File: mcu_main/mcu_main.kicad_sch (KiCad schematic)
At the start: 23 parts, among them SW1 SW_Push_Dual, SW2 SW_Push_Dual, U1 ESP32-S3-WROOM-1, U3 SGM2212-3.3, U5 SGM2212-2.8

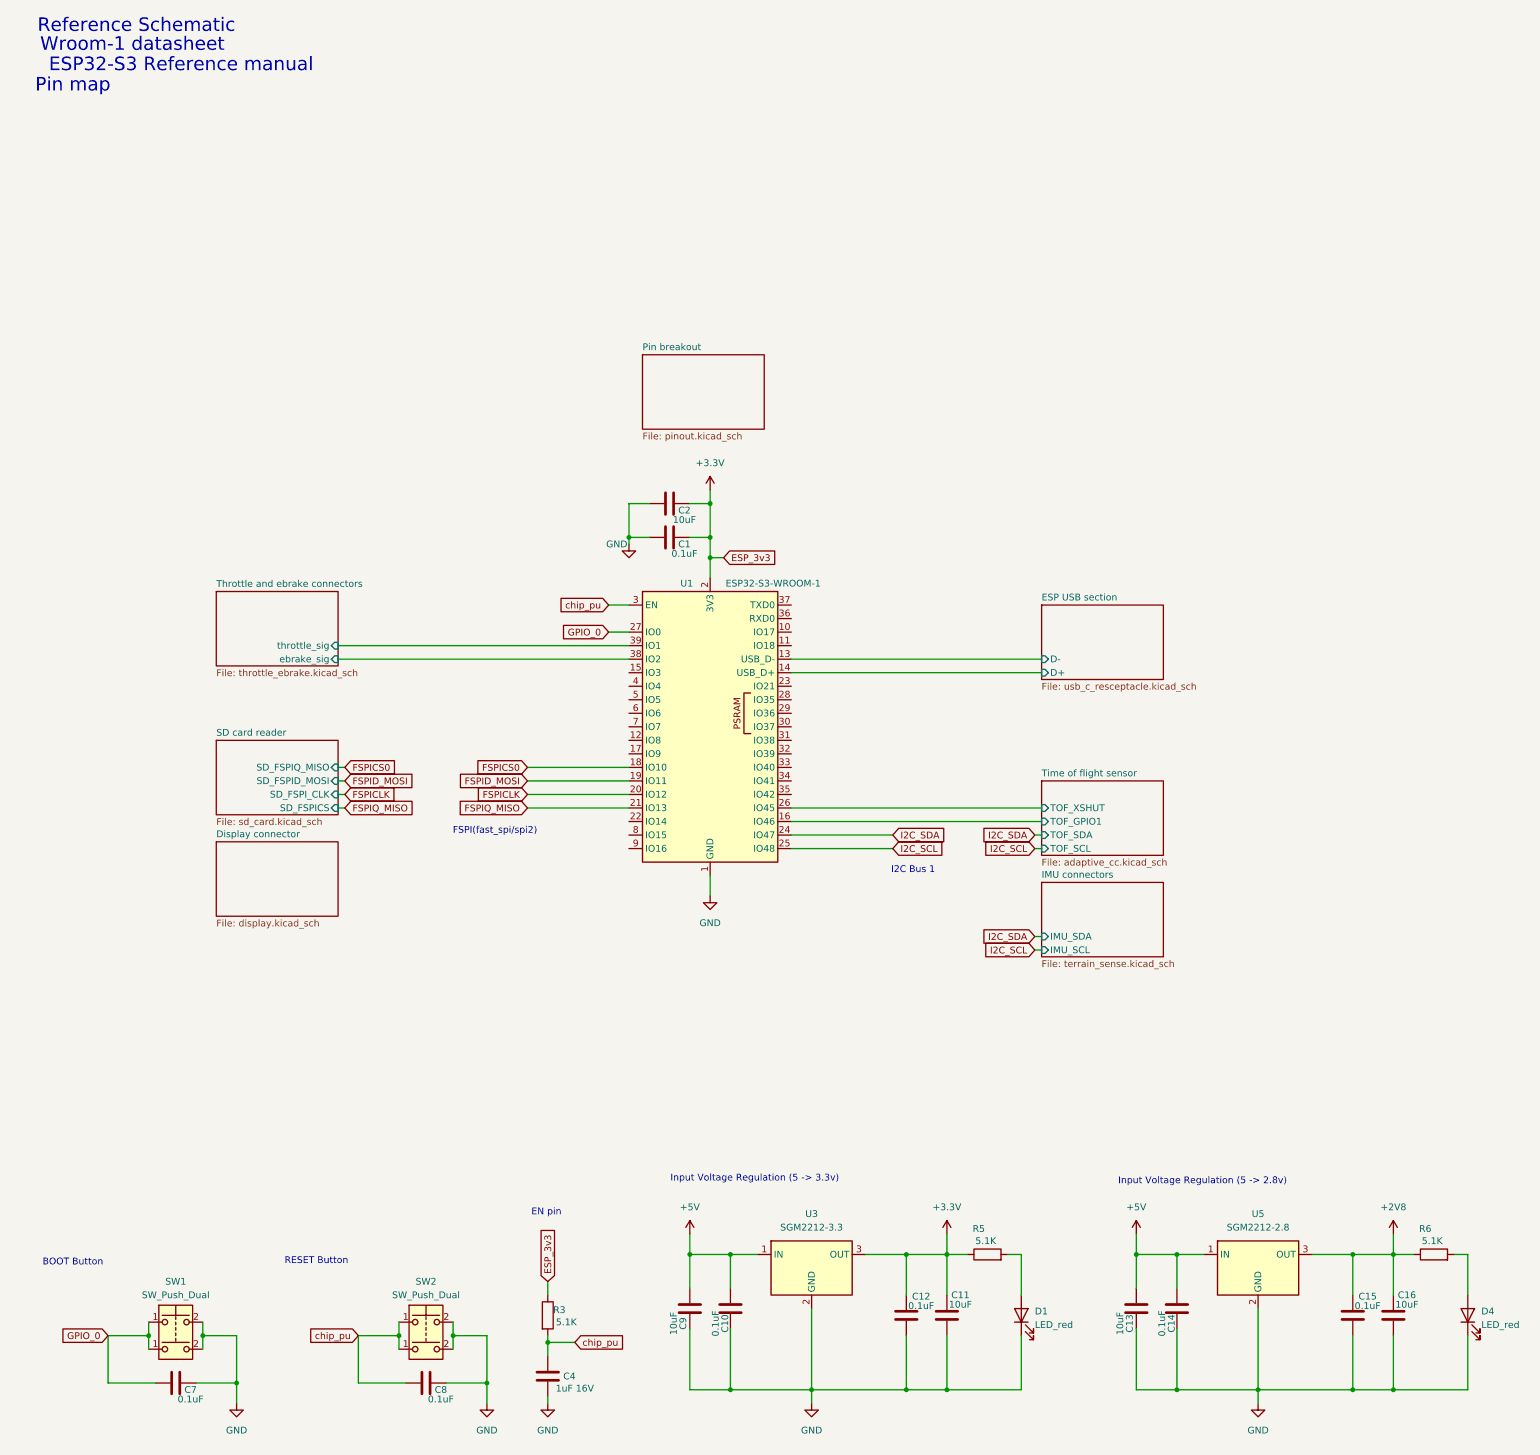
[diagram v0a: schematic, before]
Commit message: pas sensors
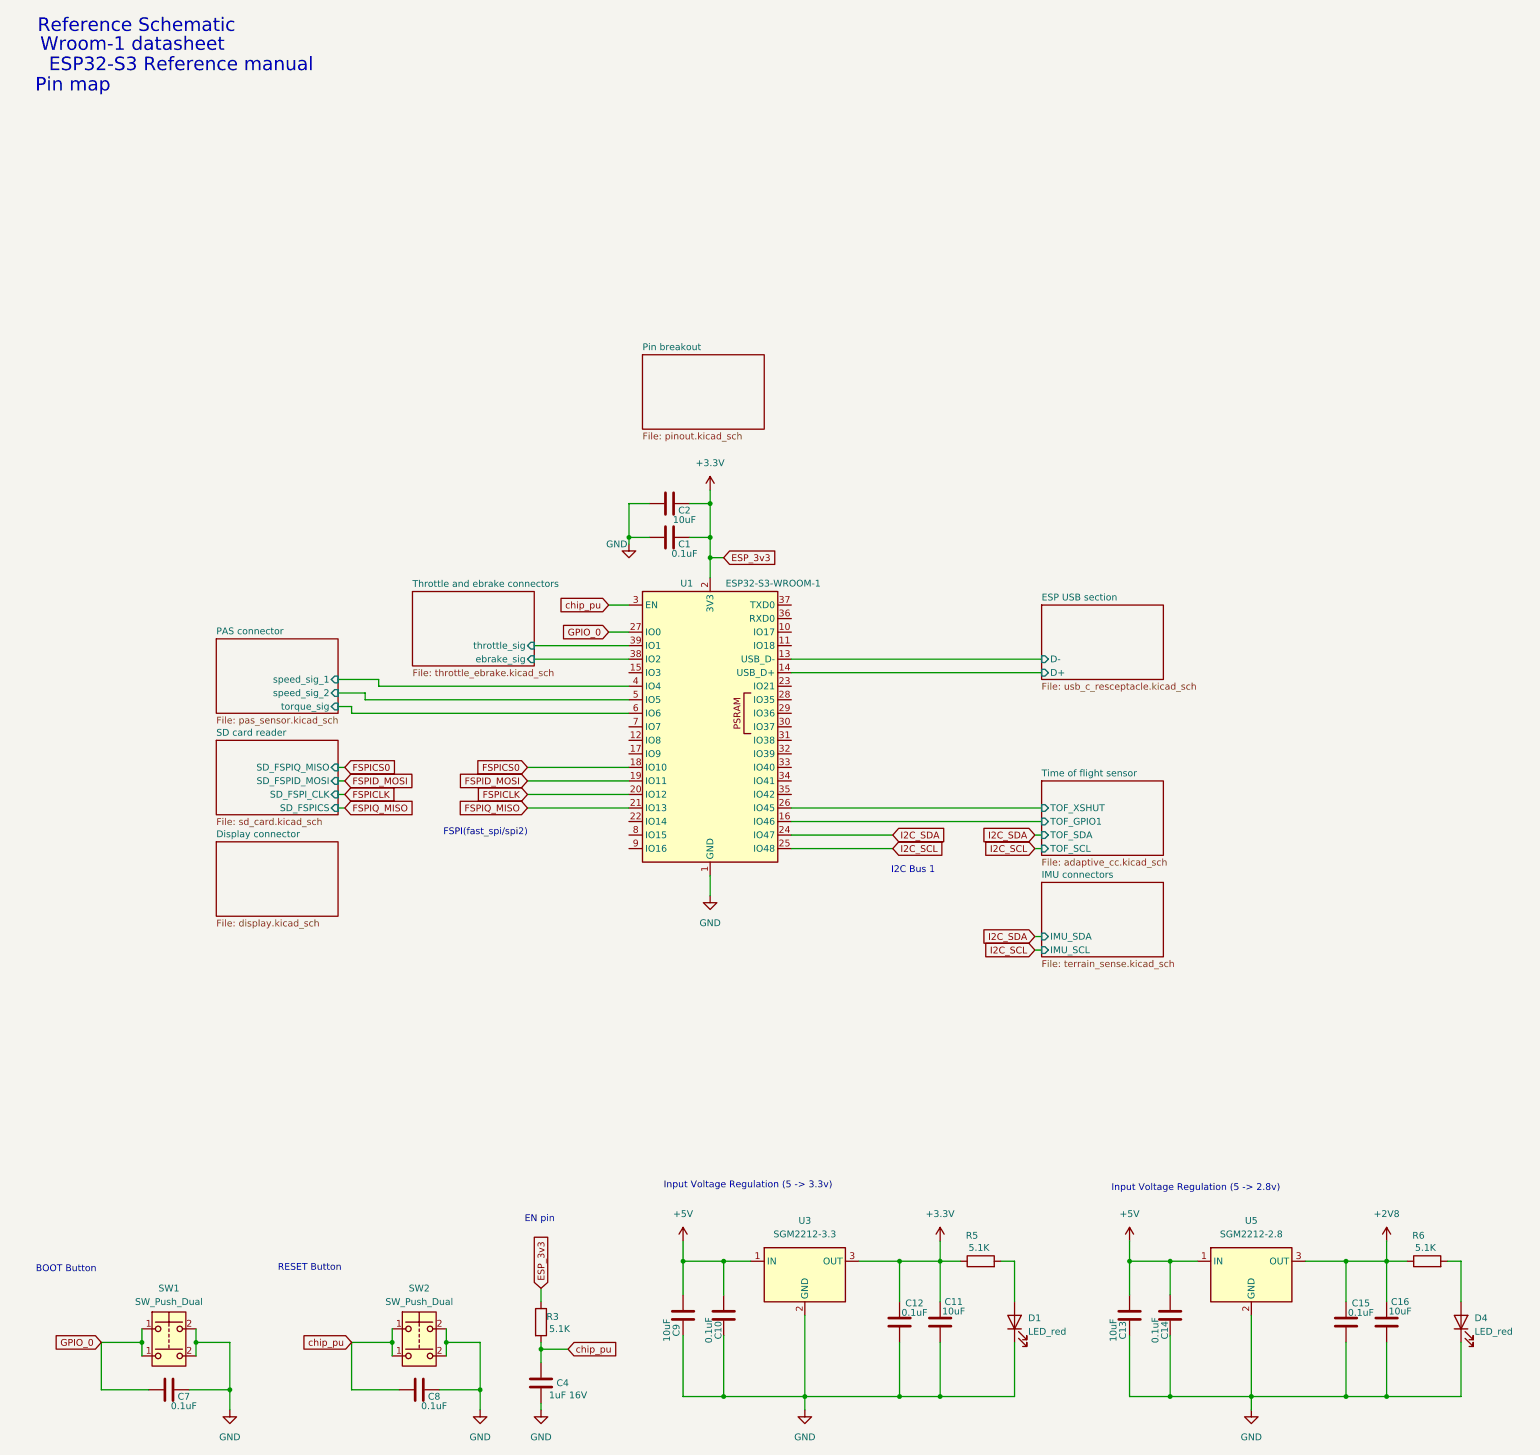
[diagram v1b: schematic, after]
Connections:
- net PAS connector/speed_sig_1: now reaches U1.4 (IO4)
- net PAS connector/speed_sig_2: now reaches U1.5 (IO5)
- net PAS connector/torque_sig: now reaches U1.6 (IO6)
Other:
- added sheet PAS connector (pas_sensor.kicad_sch)
- moved on the sheet: C10, C11, C12, C13, C14, C15, C16, C4, C7, C8, C9, D1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
